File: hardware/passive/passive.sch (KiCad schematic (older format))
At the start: 6 parts, among them J1 Main I/O, J4 Coil

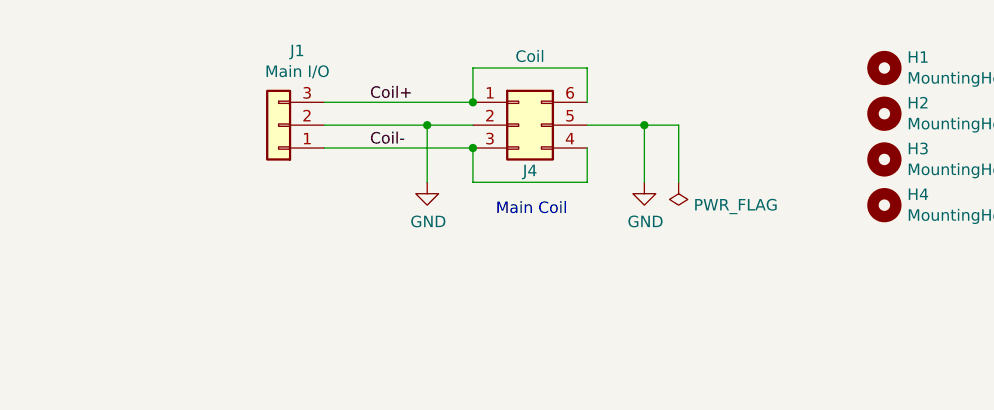
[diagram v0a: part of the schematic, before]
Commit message: passive updates
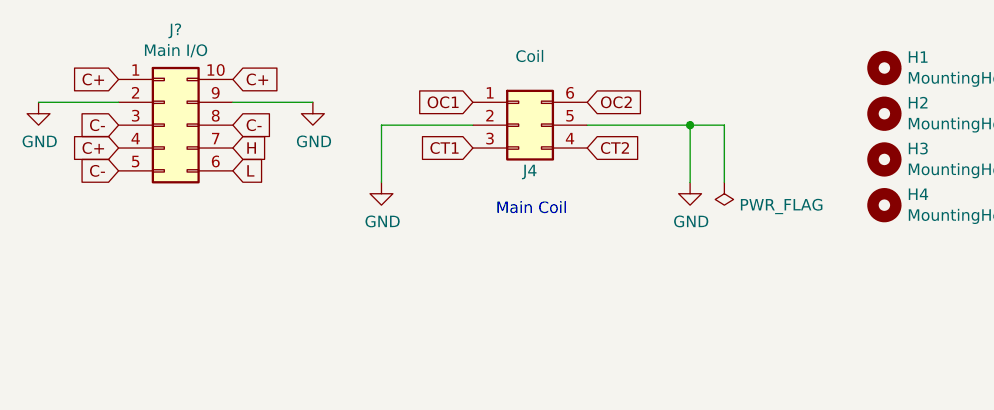
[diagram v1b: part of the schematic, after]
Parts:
- removed J1: Main I/O, cycfi_library:pin_header_1x3p_2.54mm_smd_horizontal, symbol Connector_Generic:Conn_01x03
- added J?: Main I/O, symbol Connector_Generic:Conn_02x05_Counter_Clockwise
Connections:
- net GND: now also J?.2 (Pin_2), J?.9 (Pin_9)
- net Coil+ renamed OC1
- net OC1: no longer J4.6 (Pin_6)
- net Coil- renamed CT1
- net CT1: no longer J4.4 (Pin_4)
- new net C+: J?.1 (Pin_1), J?.10 (Pin_10), J?.4 (Pin_4)
- new net C-: J?.3 (Pin_3), J?.5 (Pin_5), J?.8 (Pin_8)
- new net CT2: J4.4 (Pin_4)
- new net H: J?.7 (Pin_7)
- new net L: J?.6 (Pin_6)
- new net OC2: J4.6 (Pin_6)
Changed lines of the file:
@@
 L power:GND #PWR0101
 U 1 1 60CA6062
-P 6150 4150
-F 0 "#PWR0101" H 6150 3900 50  0001 C CNN
-F 1 "GND" H 6155 3977 50  0000 C CNN
-F 2 "" H 6150 4150 50  0001 C CNN
-F 3 "" H 6150 4150 50  0001 C CNN
-	1    6150 4150
+P 6350 4150
+F 0 "#PWR0101" H 6350 3900 50  0001 C CNN
+F 1 "GND" H 6355 3977 50  0000 C CNN
+F 2 "" H 6350 4150 50  0001 C CNN
+F 3 "" H 6350 4150 50  0001 C CNN
+	1    6350 4150
 	1    0    0    -1
 $EndComp
@@
 L power:GND #PWR0109
 U 1 1 60D40697
-P 5200 4150
-F 0 "#PWR0109" H 5200 3900 50  0001 C CNN
-F 1 "GND" H 5205 3977 50  0000 C CNN
-F 2 "" H 5200 4150 50  0001 C CNN
-F 3 "" H 5200 4150 50  0001 C CNN
-	1    5200 4150
-	1    0    0    -1
-$EndComp
-Wire Wire Line
-	5400 3900 5200 3900
+P 5000 4150
+F 0 "#PWR0109" H 5000 3900 50  0001 C CNN
+F 1 "GND" H 5005 3977 50  0000 C CNN
+F 2 "" H 5000 4150 50  0001 C CNN
+F 3 "" H 5000 4150 50  0001 C CNN
+	1    5000 4150
+	1    0    0    -1
+$EndComp
 $Bitmap
 Pos 9150 6850
@@
 $EndComp
 Wire Wire Line
-	5400 4150 5400 4000
-Wire Wire Line
-	5900 4000 5900 4150
-Wire Wire Line
-	5900 4150 5400 4150
-Wire Wire Line
-	5400 3800 5400 3650
-Wire Wire Line
-	5400 3650 5900 3650
-Wire Wire Line
-	5900 3650 5900 3800
-Wire Wire Line
-	5900 3900 6150 3900
-$Comp
-L Connector_Generic:Conn_01x03 J1
-U 1 1 60D6F0CB
-P 4550 3900
-F 0 "J1" H 4468 3575 50  0000 C CNN
-F 1 "Main I/O" H 4468 3666 50  0000 C CNN
-F 2 "cycfi_library:pin_header_1x3p_2.54mm_smd_horizontal" H 4550 3900 50  0001 C CNN
-F 3 "~" H 4550 3900 50  0001 C CNN
-	1    4550 3900
-	-1   0    0    1
-$EndComp
-Wire Wire Line
-	6150 3900 6150 4150
-Wire Wire Line
-	4750 3800 5400 3800
-Connection ~ 5400 3800
-Wire Wire Line
-	4750 3900 5200 3900
-Connection ~ 5200 3900
-Wire Wire Line
-	5200 3900 5200 4150
-Wire Wire Line
-	4750 4000 5400 4000
-Connection ~ 5400 4000
-Text Label 4950 3800 0    50   ~ 0
-Coil+
-Text Label 4950 4000 0    50   ~ 0
-Coil-
+	6350 3900 6350 4150
+Wire Wire Line
+	5000 3900 5000 4150
 $Comp
 L power:PWR_FLAG #FLG0101
 U 1 1 60D6F7D1
-P 6300 4150
-F 0 "#FLG0101" H 6300 4225 50  0001 C CNN
-F 1 "PWR_FLAG" H 6050 4250 50  0000 C CNN
-F 2 "" H 6300 4150 50  0001 C CNN
-F 3 "~" H 6300 4150 50  0001 C CNN
-	1    6300 4150
+P 6500 4150
+F 0 "#FLG0101" H 6500 4225 50  0001 C CNN
+F 1 "PWR_FLAG" H 6250 4250 50  0000 C CNN
+F 2 "" H 6500 4150 50  0001 C CNN
+F 3 "~" H 6500 4150 50  0001 C CNN
+	1    6500 4150
 	-1   0    0    1
 $EndComp
 Wire Wire Line
-	6300 4150 6300 3900
-Wire Wire Line
-	6300 3900 6150 3900
-Connection ~ 6150 3900
+	6500 4150 6500 3900
+Wire Wire Line
+	6500 3900 6350 3900
+Connection ~ 6350 3900
+$Comp
+L Connector_Generic:Conn_02x05_Counter_Clockwise J?
+U 1 1 60FA7E20
+P 4050 3900
+F 0 "J?" H 4100 4317 50  0000 C CNN
+F 1 "Main I/O" H 4100 4226 50  0000 C CNN
+F 2 "" H 4050 3900 50  0001 C CNN
+F 3 "~" H 4050 3900 50  0001 C CNN
+	1    4050 3900
+	1    0    0    -1
+$EndComp
+Text GLabel 3850 3700 0    50   Input ~ 0
+C+
+$Comp
+L power:GND #PWR?
+U 1 1 60FA9CE2
+P 3500 3800
+F 0 "#PWR?" H 3500 3550 50  0001 C CNN
+F 1 "GND" H 3505 3627 50  0000 C CNN
+F 2 "" H 3500 3800 50  0001 C CNN
+F 3 "" H 3500 3800 50  0001 C CNN
+	1    3500 3800
+	1    0    0    -1
+$EndComp
+Text GLabel 4350 3700 2    50   Input ~ 0
+C+
+Text GLabel 3850 3900 0    50   Input ~ 0
+C-
+Text GLabel 4350 3900 2    50   Input ~ 0
+C-
+$Comp
+L power:GND #PWR?
+U 1 1 60FAABF1
+P 4700 3800
+F 0 "#PWR?" H 4700 3550 50  0001 C CNN
+F 1 "GND" H 4705 3627 50  0000 C CNN
+F 2 "" H 4700 3800 50  0001 C CNN
+F 3 "" H 4700 3800 50  0001 C CNN
+	1    4700 3800
+	1    0    0    -1
+$EndComp
+Wire Wire Line
+	3500 3800 3850 3800
+Wire Wire Line
+	4350 3800 4700 3800
+Text GLabel 3850 4000 0    50   Input ~ 0
+C+
+Text GLabel 3850 4100 0    50   Input ~ 0
+C-
+Text GLabel 4350 4000 2    50   Input ~ 0
+H
+Text GLabel 4350 4100 2    50   Input ~ 0
+L
+Wire Wire Line
+	5000 3900 5400 3900
+Wire Wire Line
+	5900 3900 6350 3900
+Text GLabel 5400 3800 0    50   Input ~ 0
+OC1
+Text GLabel 5900 3800 2    50   Input ~ 0
+OC2
+Text GLabel 5400 4000 0    50   Input ~ 0
+CT1
+Text GLabel 5900 4000 2    50   Input ~ 0
+CT2
 $EndSCHEMATC
